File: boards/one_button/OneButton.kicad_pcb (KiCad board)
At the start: 2 copper layers, 20 x 20 mm, 18 parts, among them J1 INPUT, J2 OUTPUT, SW1 TS-1187A-B-A-B, U1 CH32V003F4U6

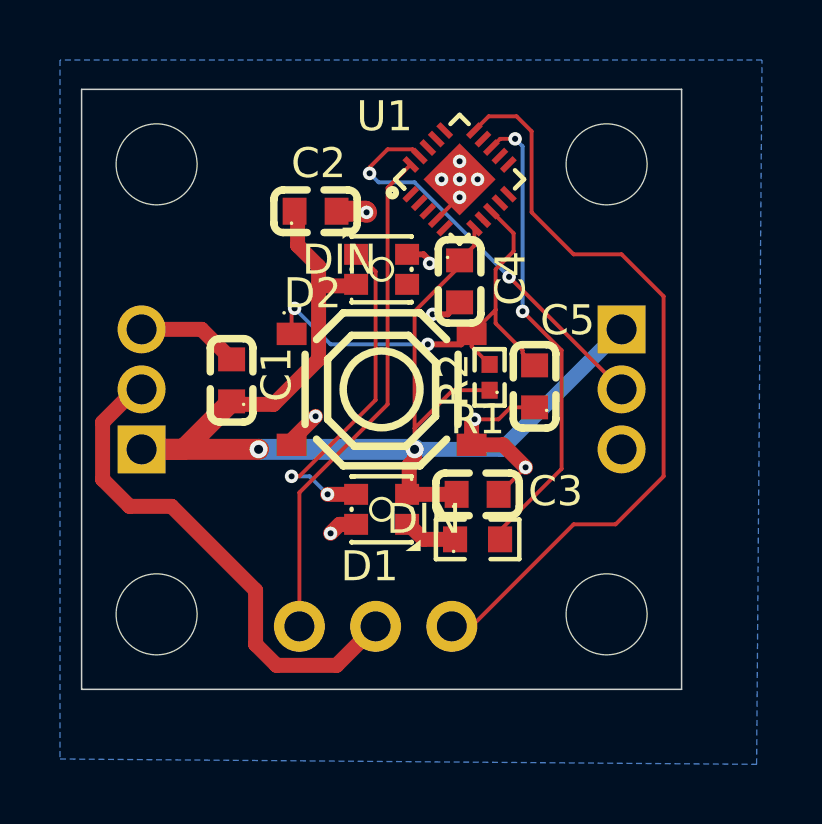
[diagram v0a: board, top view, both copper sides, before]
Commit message: Update step models
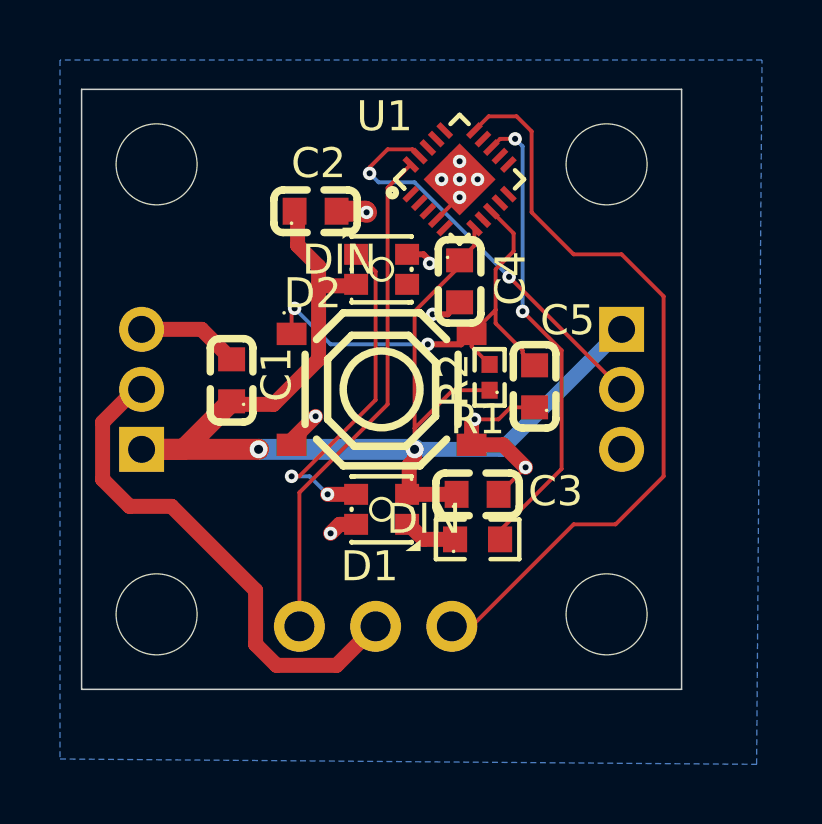
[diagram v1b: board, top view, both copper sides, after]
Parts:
- J1, J2: footprint easyeda2kicad:CONN-TH_B3B-PH-K-S -> easyeda2kicad:CONN-TH_3P-P2.00_S3B-PH-K-S-LF-SN
- turned J1 to 90 degrees
- turned J2 to -90 degrees
